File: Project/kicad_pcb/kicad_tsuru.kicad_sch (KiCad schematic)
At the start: 81 parts, among them J1 USB_C_Receptacle_USB2.0, J2 Conn_ARM_SWD_TagConnect_TC203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, J3 Conn_01x05_Pin, SW1 RotaryEncoder_Switch, U2 AP2112K-3.3, U2 PRTR5V0U2X, U3 STM32F072C8Tx

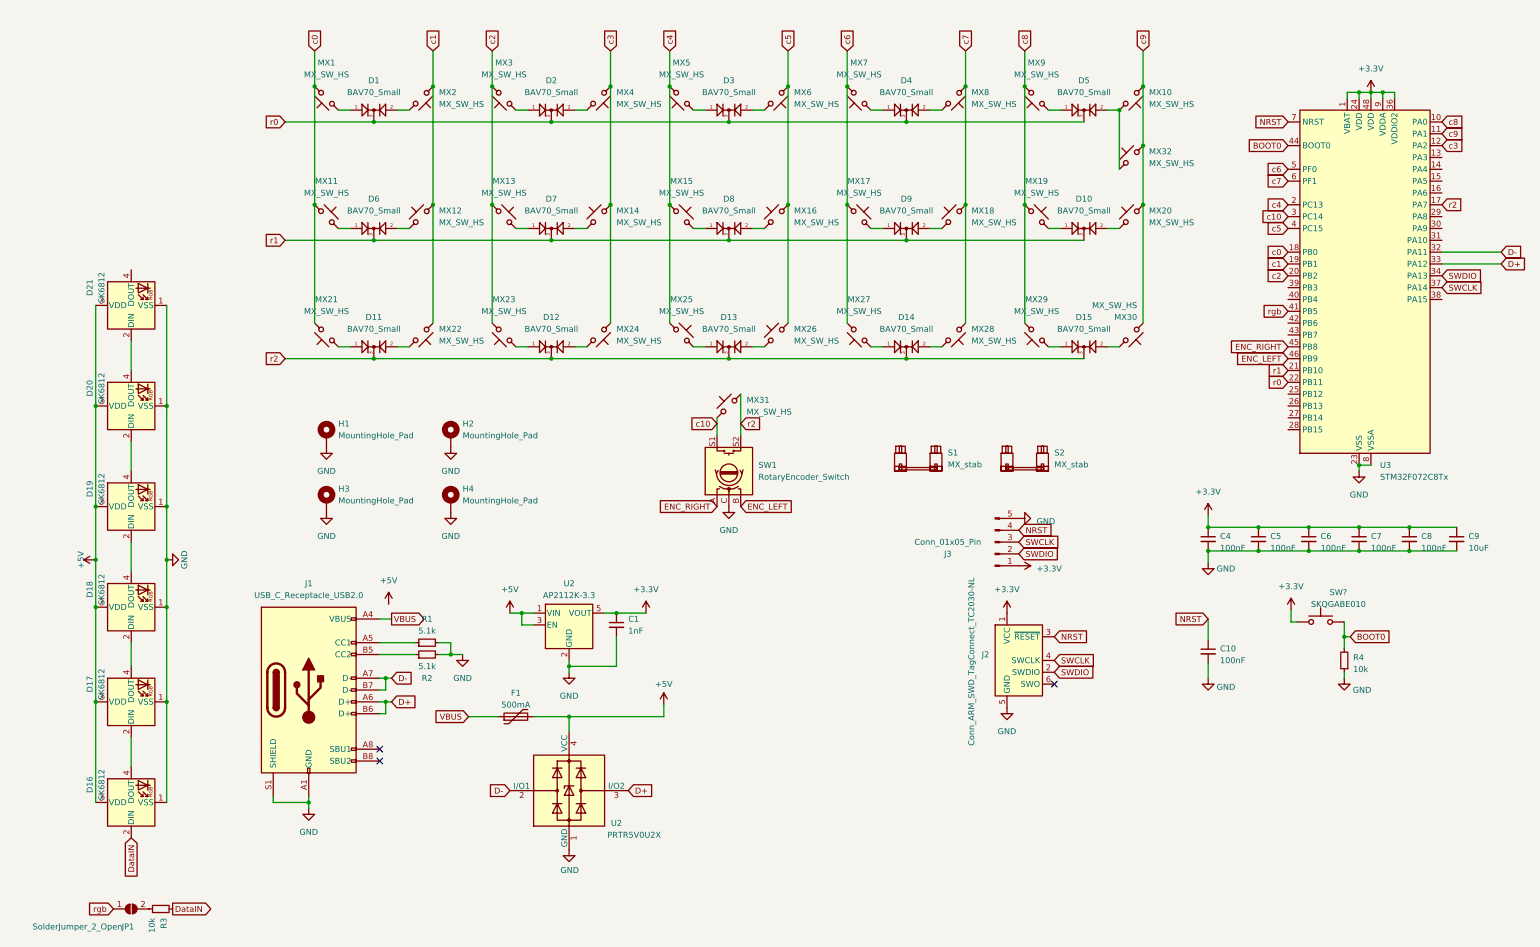
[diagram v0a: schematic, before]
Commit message: readme update
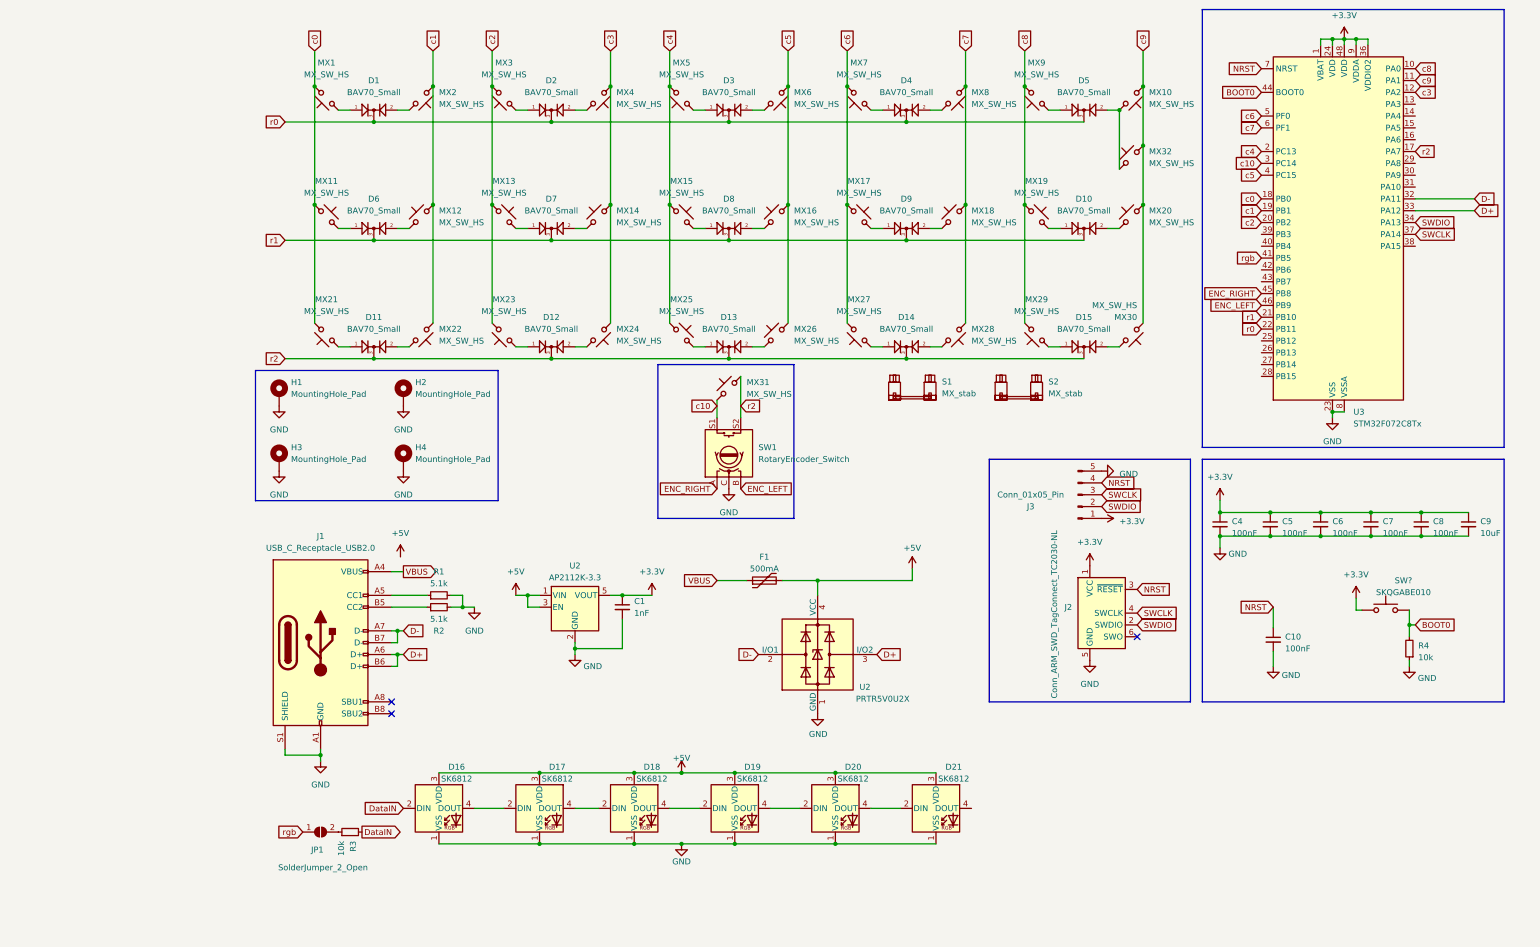
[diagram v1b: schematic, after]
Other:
- moved on the sheet: C1, C10, C4, C5, C6, C7, C8, C9, D16, D17, D18, D19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
